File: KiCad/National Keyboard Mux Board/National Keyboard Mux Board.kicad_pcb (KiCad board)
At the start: 2 copper layers, 80 x 37.5 mm, 43 parts, among them J1 Conn_01x01_Female, J10 Conn_01x01_Female, J11 Conn_01x01_Female, J12 Conn_01x01_Female, J13 Conn_01x01_Female, J14 Conn_01x01_Female, J15 Conn_01x01_Female, J16 Conn_01x01_Female, J17 Conn_01x01_Female, J18 Conn_01x01_Female, J19 Conn_02x08_Odd_Even, J2 Conn_01x01_Female, J3 Conn_01x01_Female, J4 Conn_01x01_Female, J5 Conn_01x01_Female, J6 Conn_01x01_Female, J7 Conn_01x01_Female, J8 Conn_01x01_Female, J9 Conn_01x01_Female

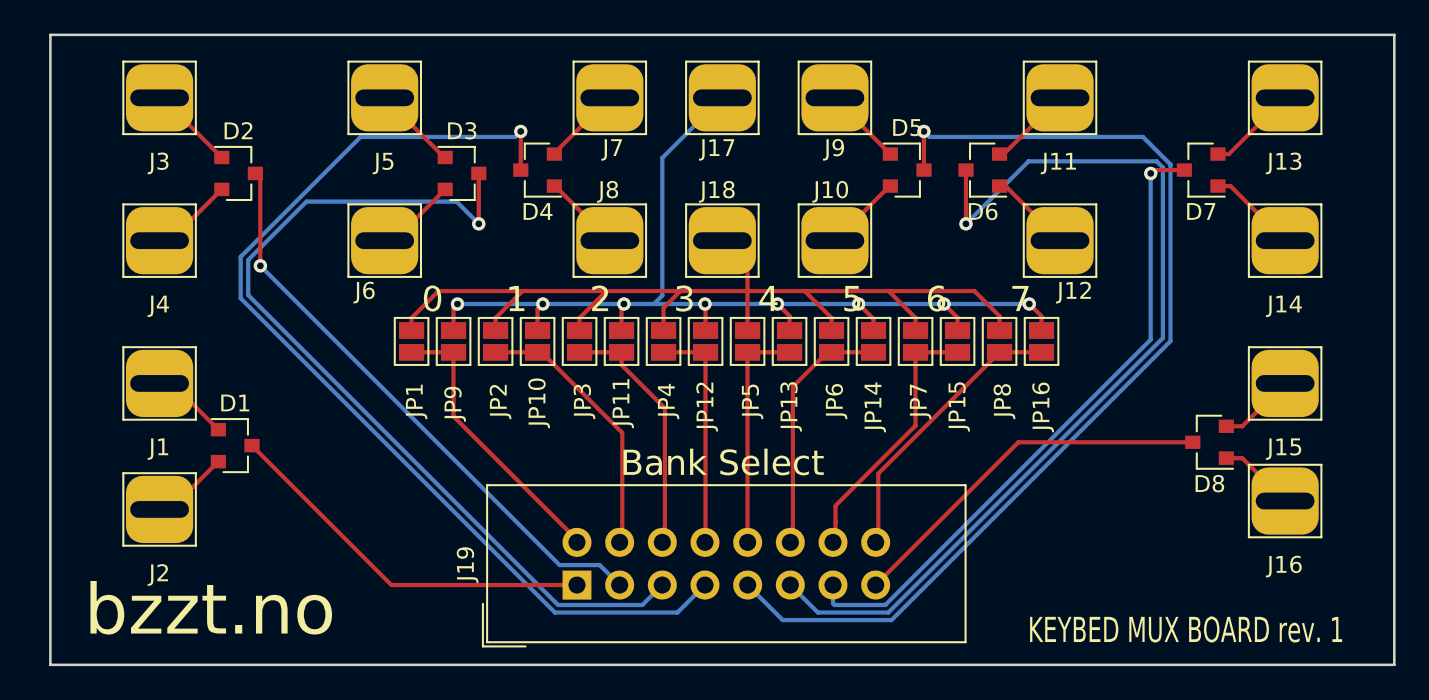
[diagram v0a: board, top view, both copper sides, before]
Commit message: more work towards production
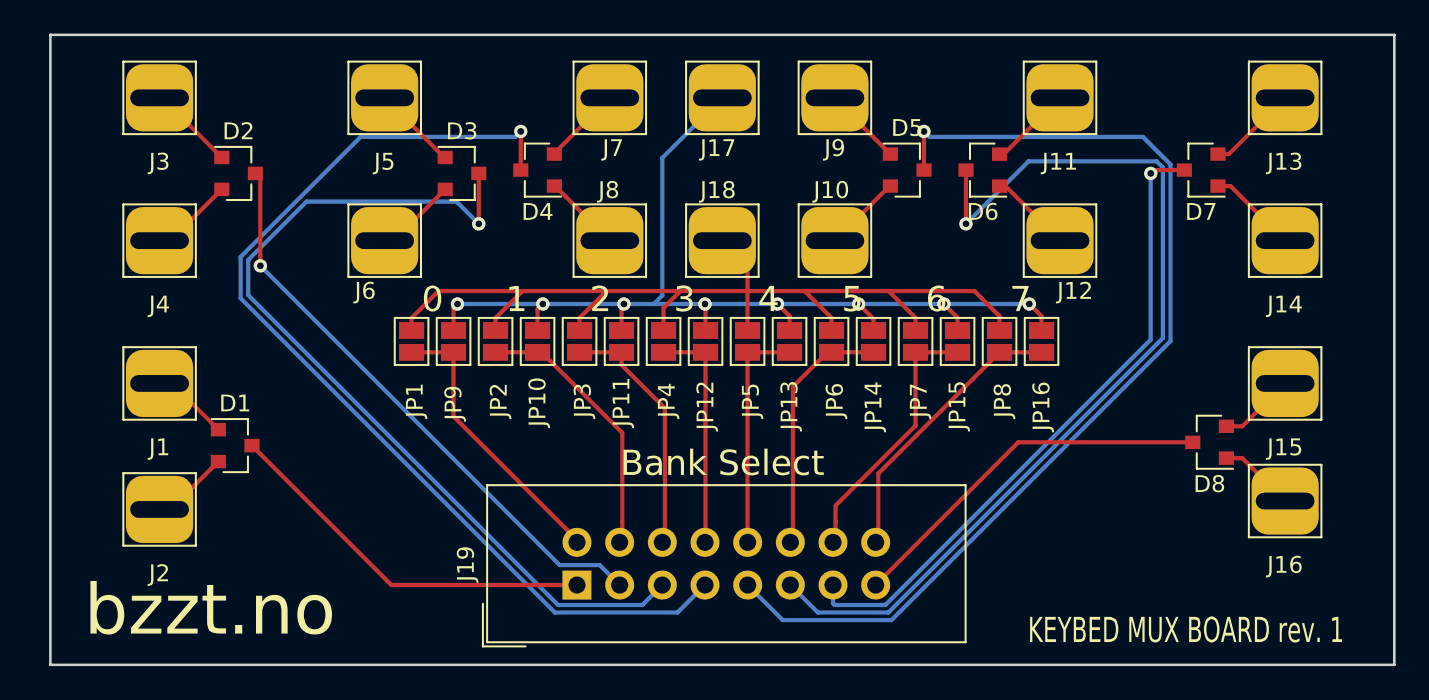
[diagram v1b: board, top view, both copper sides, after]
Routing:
- added copper zone on B.Cu, net (none)
- added copper zone on F.Cu, net (none)
